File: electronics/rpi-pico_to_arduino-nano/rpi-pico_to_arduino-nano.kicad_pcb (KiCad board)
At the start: 2 copper layers, 2 parts, among them U1 Pico

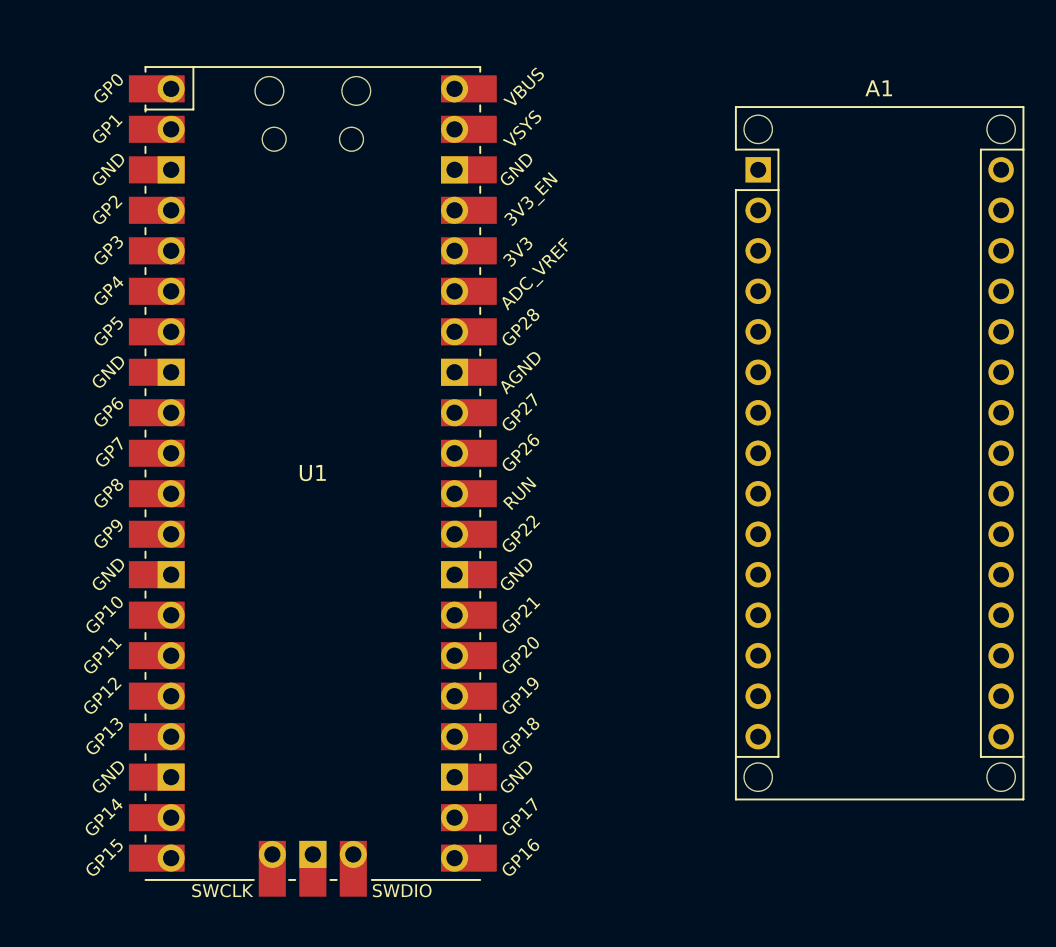
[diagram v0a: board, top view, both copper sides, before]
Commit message: add some connections and comments
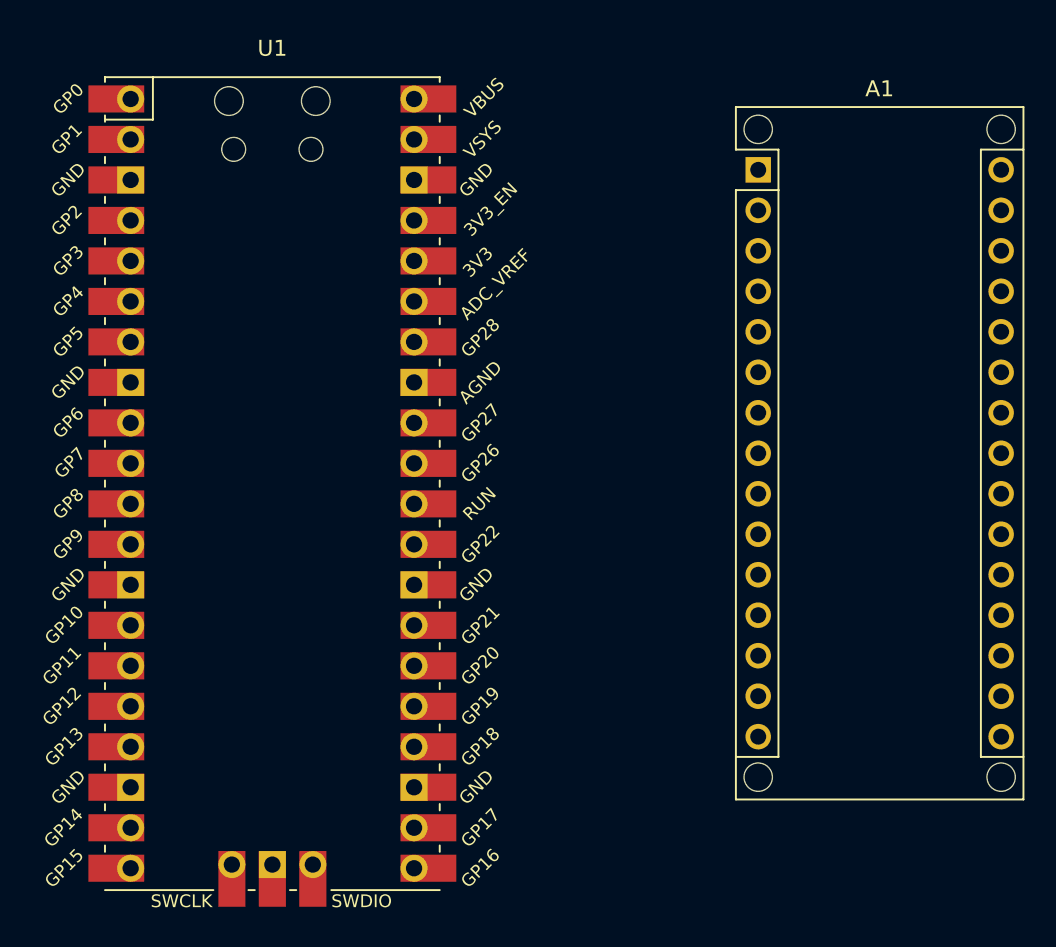
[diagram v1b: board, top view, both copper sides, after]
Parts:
- moved U1 2.62 mm to (153.7, 107.3)
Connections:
- A1 pad 1: unconnected-(A1-Pad1) -> /GPIO1
- A1 pad 10: unconnected-(A1-Pad10) -> /GPIO7
- A1 pad 11: unconnected-(A1-Pad11) -> /GPIO8
- A1 pad 12: unconnected-(A1-Pad12) -> /GPIO9
- A1 pad 13: unconnected-(A1-Pad13) -> /GPIO10
- A1 pad 14: unconnected-(A1-Pad14) -> /GPIO11
- A1 pad 15: unconnected-(A1-Pad15) -> /GPIO12
- A1 pad 16: unconnected-(A1-Pad16) -> /GPIO13
- A1 pad 19: unconnected-(A1-Pad19) -> /GPIO26_ADC0
- A1 pad 2: unconnected-(A1-Pad2) -> /GPIO0
- A1 pad 20: unconnected-(A1-Pad20) -> /GPIO27_ADC1
- A1 pad 21: unconnected-(A1-Pad21) -> /GPIO26_ADC0
- A1 pad 29: unconnected-(A1-Pad29) -> GND
- A1 pad 4: unconnected-(A1-Pad4) -> GND
- A1 pad 5: unconnected-(A1-Pad5) -> /GPIO2
- A1 pad 6: unconnected-(A1-Pad6) -> /GPIO3
- A1 pad 7: unconnected-(A1-Pad7) -> /GPIO4
- A1 pad 8: unconnected-(A1-Pad8) -> /GPIO5
- A1 pad 9: unconnected-(A1-Pad9) -> /GPIO6
- U1 pad 1: unconnected-(U1-Pad1) -> /GPIO0
- U1 pad 10: unconnected-(U1-Pad10) -> /GPIO7
- U1 pad 11: unconnected-(U1-Pad11) -> /GPIO8
- U1 pad 12: unconnected-(U1-Pad12) -> /GPIO9
- U1 pad 13: unconnected-(U1-Pad13) -> GND
- U1 pad 14: unconnected-(U1-Pad14) -> /GPIO10
- U1 pad 15: unconnected-(U1-Pad15) -> /GPIO11
- U1 pad 16: unconnected-(U1-Pad16) -> /GPIO12
- U1 pad 17: unconnected-(U1-Pad17) -> /GPIO13
- U1 pad 18: unconnected-(U1-Pad18) -> GND
- U1 pad 19: unconnected-(U1-Pad19) -> /GPIO14
- U1 pad 2: unconnected-(U1-Pad2) -> /GPIO1
- U1 pad 20: unconnected-(U1-Pad20) -> /GPIO15
- U1 pad 21: unconnected-(U1-Pad21) -> /GPIO16
- U1 pad 22: unconnected-(U1-Pad22) -> /GPIO17
- U1 pad 23: unconnected-(U1-Pad23) -> GND
- U1 pad 24: unconnected-(U1-Pad24) -> /GPIO18
- U1 pad 25: unconnected-(U1-Pad25) -> /GPIO19
- U1 pad 26: unconnected-(U1-Pad26) -> /GPIO20
- U1 pad 27: unconnected-(U1-Pad27) -> /GPIO21
- U1 pad 28: unconnected-(U1-Pad28) -> GND
- U1 pad 29: unconnected-(U1-Pad29) -> /GPIO22
- U1 pad 3: unconnected-(U1-Pad3) -> GND
- U1 pad 30: unconnected-(U1-Pad30) -> /RUN
- U1 pad 31: unconnected-(U1-Pad31) -> /GPIO26_ADC0
- U1 pad 32: unconnected-(U1-Pad32) -> /GPIO27_ADC1
- U1 pad 33: unconnected-(U1-Pad33) -> GND
- U1 pad 34: unconnected-(U1-Pad34) -> /GPIO28_ADC2
- U1 pad 35: unconnected-(U1-Pad35) -> /ADC_VREF
- U1 pad 36: unconnected-(U1-Pad36) -> /3V3
- U1 pad 37: unconnected-(U1-Pad37) -> /3V3_EN
- U1 pad 38: unconnected-(U1-Pad38) -> GND
- U1 pad 39: unconnected-(U1-Pad39) -> /VSYS
- U1 pad 4: unconnected-(U1-Pad4) -> /GPIO2
- U1 pad 40: unconnected-(U1-Pad40) -> /VBUS
- U1 pad 41: unconnected-(U1-Pad41) -> /SWCLK
- U1 pad 42: unconnected-(U1-Pad42) -> GND
- U1 pad 43: unconnected-(U1-Pad43) -> /SWDIO
- U1 pad 5: unconnected-(U1-Pad5) -> /GPIO3
- U1 pad 6: unconnected-(U1-Pad6) -> /GPIO4
- U1 pad 7: unconnected-(U1-Pad7) -> /GPIO5
- U1 pad 8: unconnected-(U1-Pad8) -> GND
- U1 pad 9: unconnected-(U1-Pad9) -> /GPIO6
